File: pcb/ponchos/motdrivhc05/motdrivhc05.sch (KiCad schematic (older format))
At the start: 22 parts

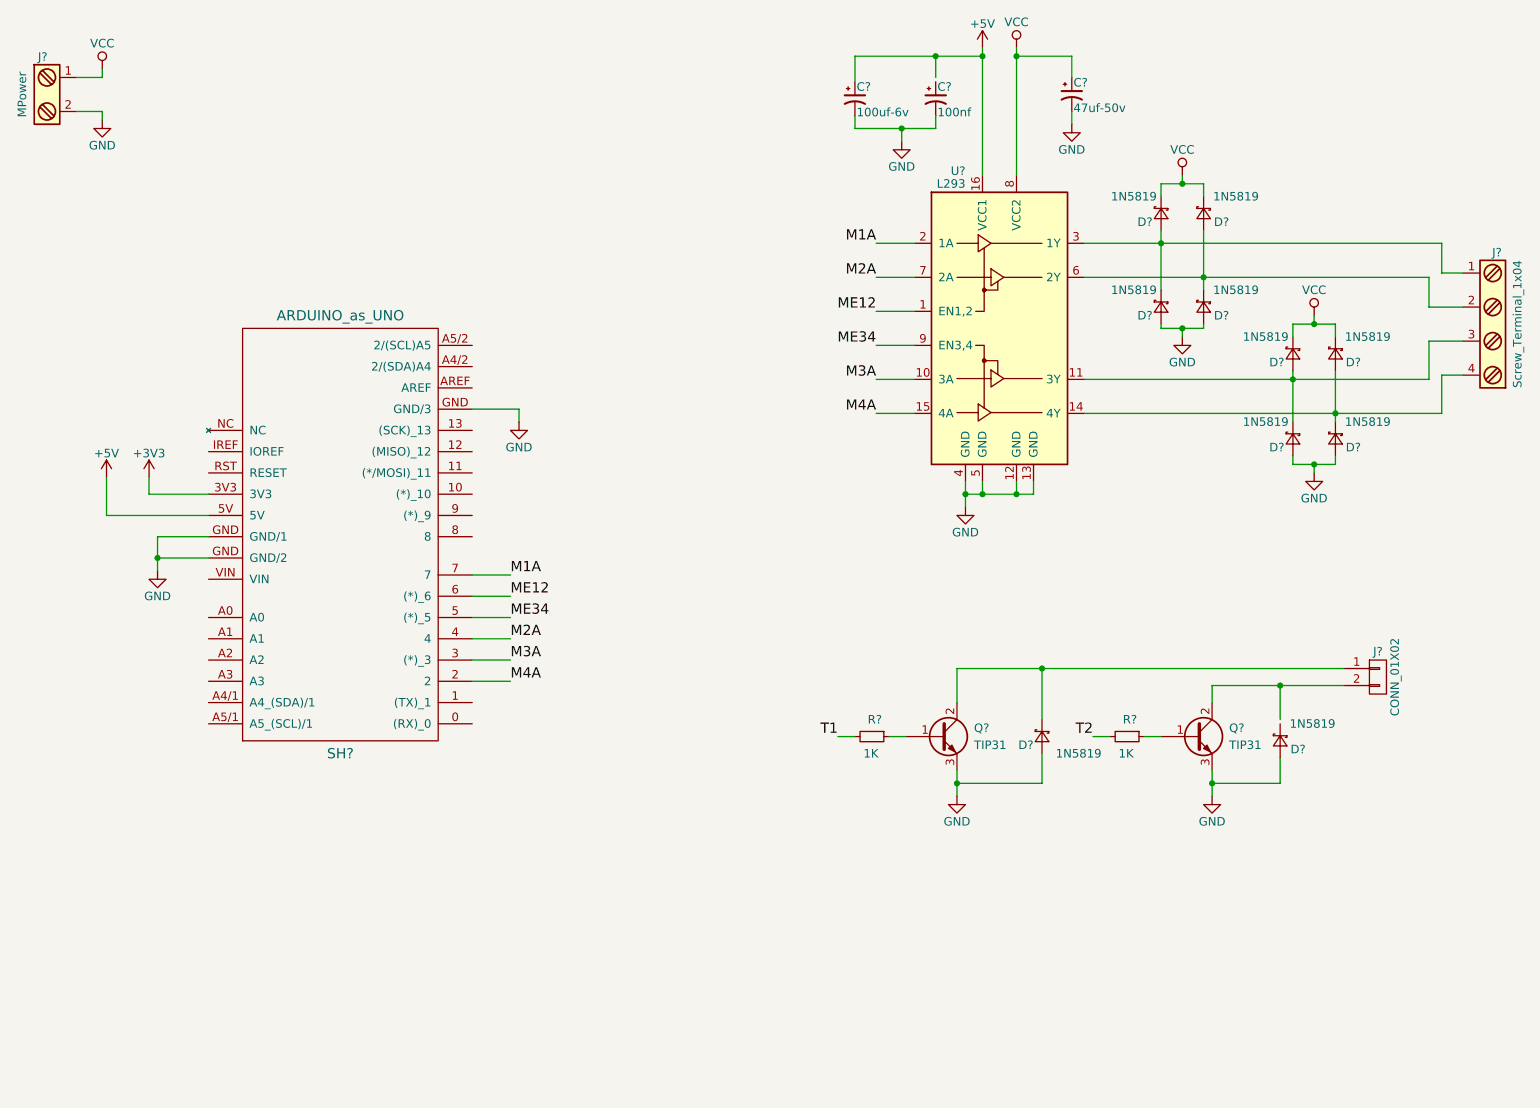
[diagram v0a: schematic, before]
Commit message: En proceso...
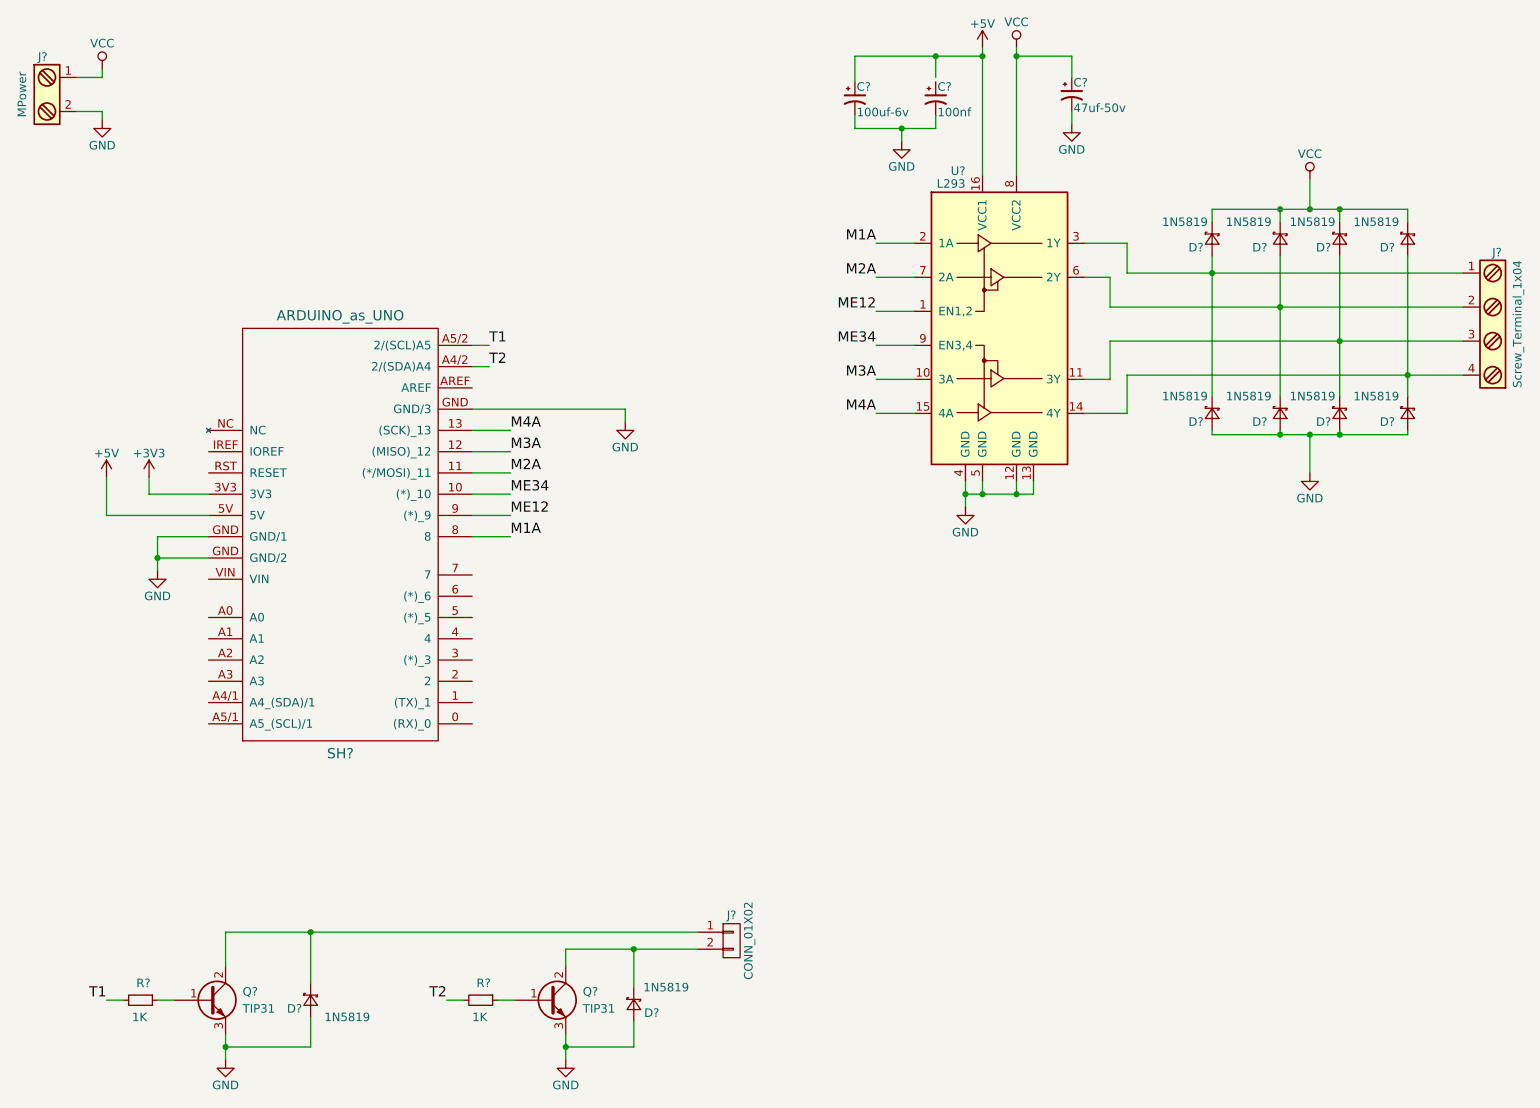
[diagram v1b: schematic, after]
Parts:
- removed D? (x6): 1N5819, symbol D_Schottky_Small
- added D? (x6): 1N5819, symbol D_Schottky_Small
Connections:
- net GND: now also D?.2 (A), D?.2 (A)
- net M1A: now also SH?.8; no longer SH?.7
- net M2A: now also SH?.11 ((*/MOSI)_11); no longer SH?.4
- net M3A: now also SH?.12 ((MISO)_12); no longer SH?.3 ((*)_3)
- net M4A: now also SH?.13 ((SCK)_13); no longer SH?.2
- net ME12: now also SH?.9 ((*)_9); no longer SH?.6 ((*)_6)
- net ME34: now also SH?.10 ((*)_10); no longer SH?.5 ((*)_5)
- net T1: now also SH?.A5/2 (2/(SCL)A5)
- net T2: now also SH?.A4/2 (2/(SDA)A4)
- net VCC: now also D?.1 (K), D?.1 (K), D?.1 (K), D?.1 (K)
- net at D?.1 (K), J?.1, U?.3 (1Y): now also D?.2 (A)
- net at D?.1 (K), J?.2, U?.6 (2Y): now also D?.2 (A)
- net at J?.3, U?.11 (3Y): now also D?.1 (K), D?.2 (A)
- net at J?.4, U?.14 (4Y): now also D?.1 (K), D?.2 (A)
- net at J?.2 (P2), Q?.2 (C): now also D?.1 (K)
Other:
- moved on the sheet: D?, J?, Q?, R?
